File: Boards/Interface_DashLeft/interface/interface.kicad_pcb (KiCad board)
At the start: 2 copper layers, 83.8 x 53.3 mm, 7 parts, among them J1 UF_2_VT, J2 MM_F_VT_08, J3 Ampseal_23_VT, J4 MM_F_VT_04, J5 MM_F_VT_20, U1 RJ45_VT

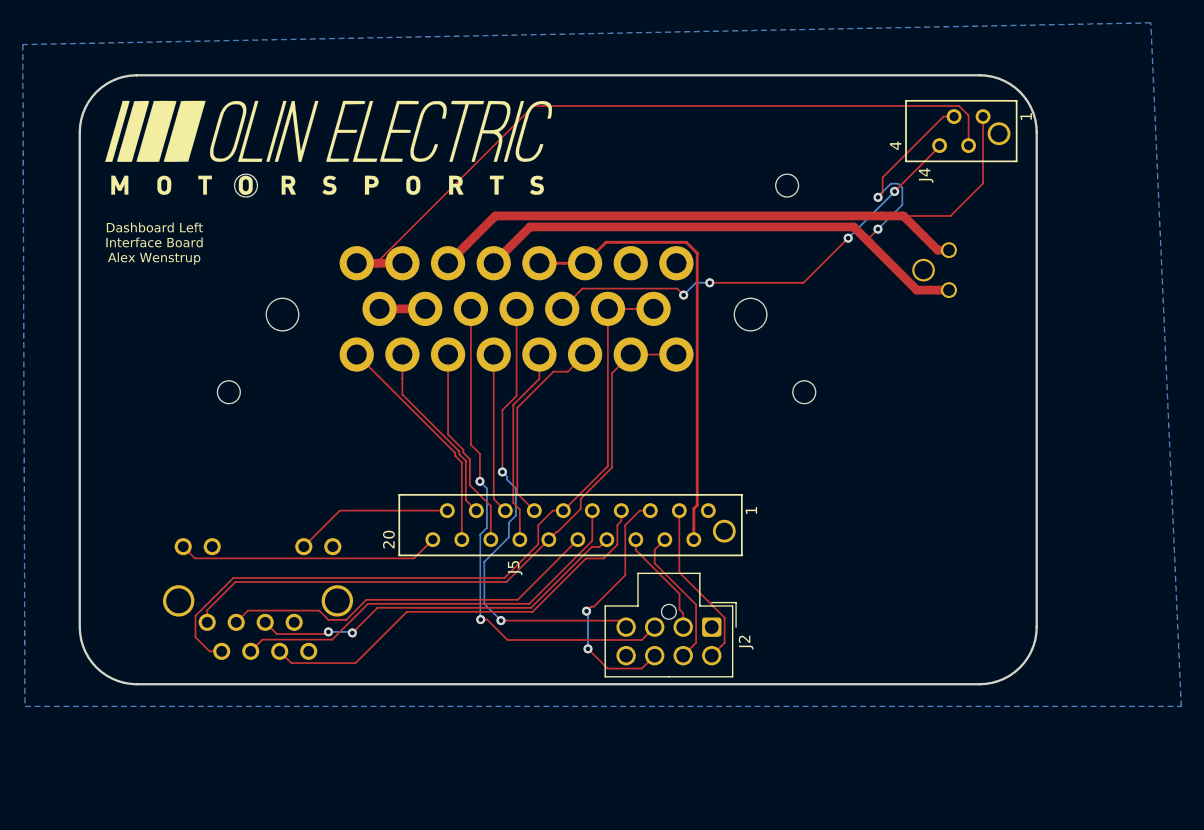
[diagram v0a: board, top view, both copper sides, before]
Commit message: Rev1 dashleft layout gerbers
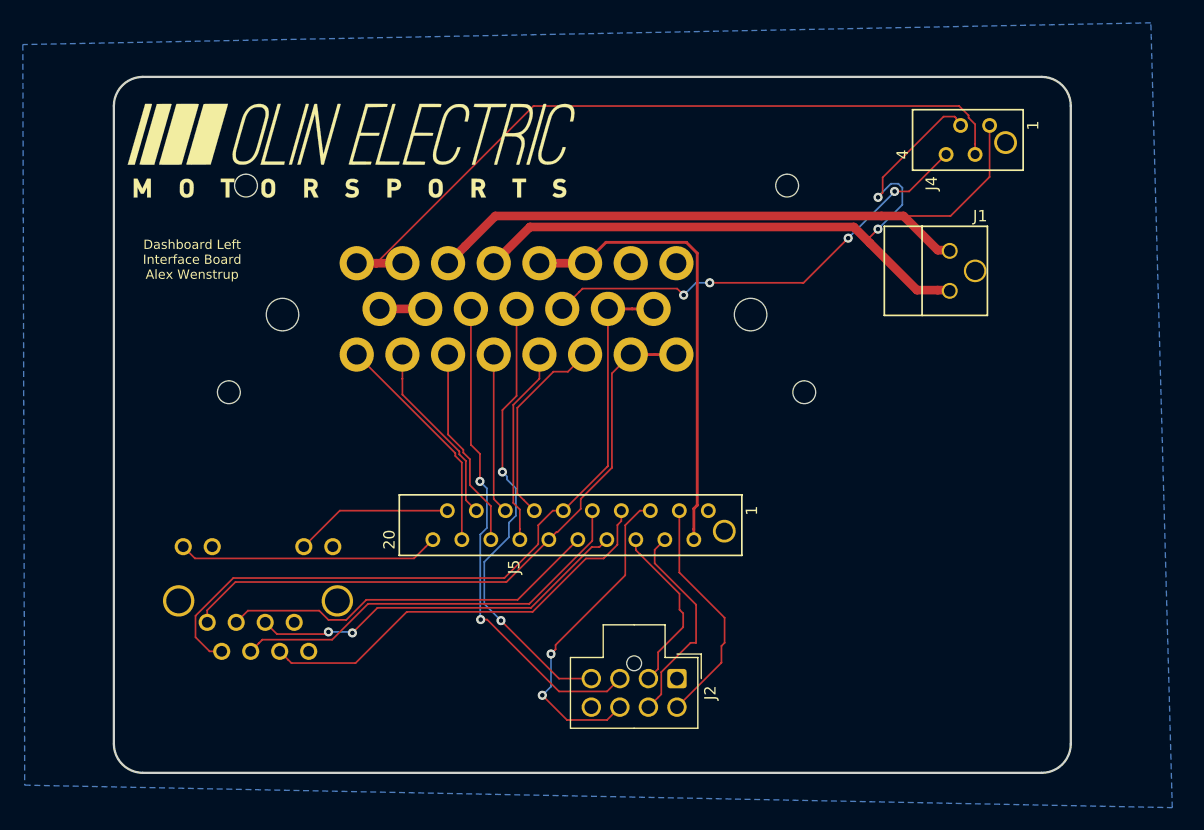
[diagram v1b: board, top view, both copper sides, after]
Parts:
- J1: moved to F.Cu
- moved J2 5.44 mm to (62.9, 119.8)
- moved G*** 1.98 mm to (34.4, 73.5)
- moved J4 0.96 mm to (85.2, 71.3)
- moved J1 0.09 mm to (86.8, 82.3), turned to 0 degrees
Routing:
- net /Drive_Select-: track 22.2 -> 28.8 mm
- net /Drive_Select_Sense: track 12.5 -> 18.6 mm
- net /5V: track 9.59 -> 15.4 mm
- net /Drive_Select+: track 15.3 -> 21.1 mm
- net /SCL: track 41.3 -> 40.1 mm
- net /SDA: track 44.8 -> 43.6 mm
- net /ESTOP->HVD: track 62.7 -> 63.7 mm
- net /IS->BOTS: track 64.8 -> 65.8 mm
- net /BOTS->ESTOP: track 62.8 -> 62.2 mm
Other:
- board size 83.8 x 53.3 mm -> 83.8 x 61 mm
